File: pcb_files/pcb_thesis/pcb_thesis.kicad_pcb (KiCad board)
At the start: 2 copper layers, 22 parts, among them J1 goldpin 1x6, J2 goldpin 1x2, J3 goldpin 1x2, Q1 PNP, SW1 RESET SW, SW3 ACTION SW, U1 ATmega32L-8AU, Y1 8MHz

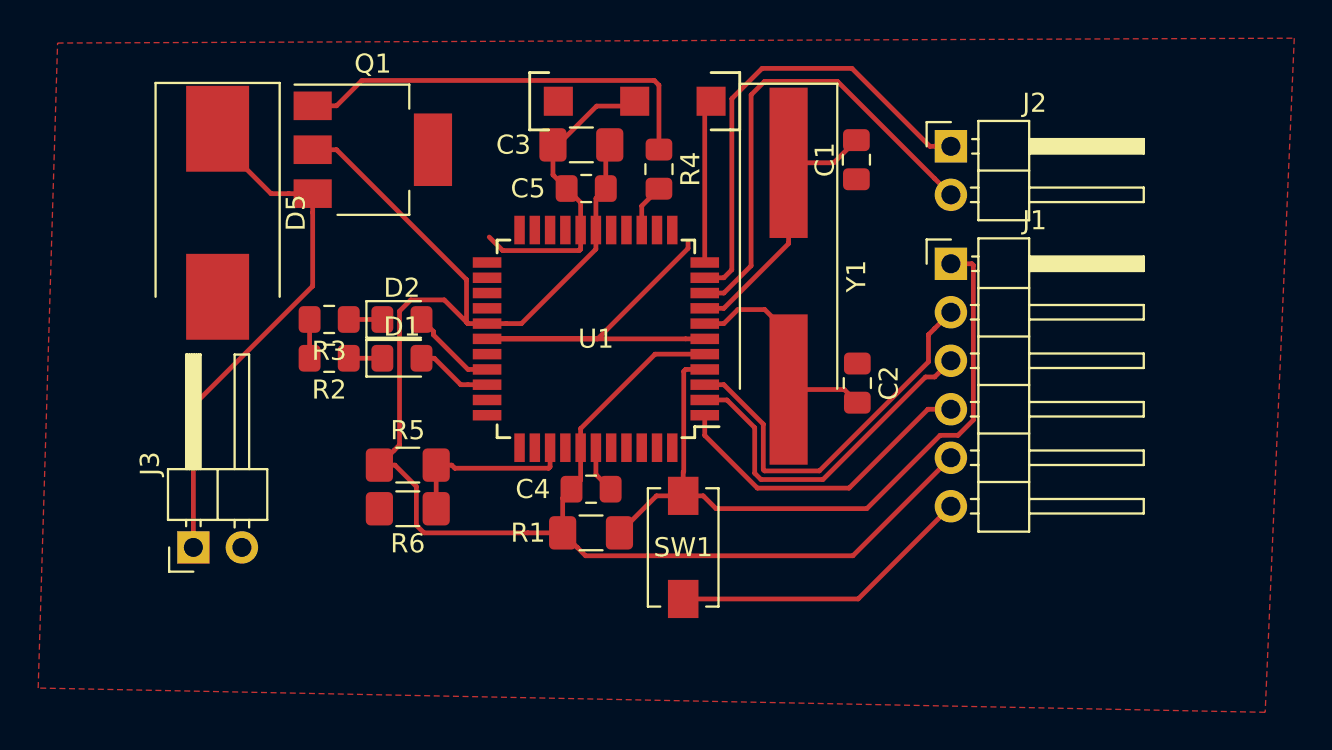
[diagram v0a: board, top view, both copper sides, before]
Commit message: Przygotowanie plikow do wytrawiania plytki
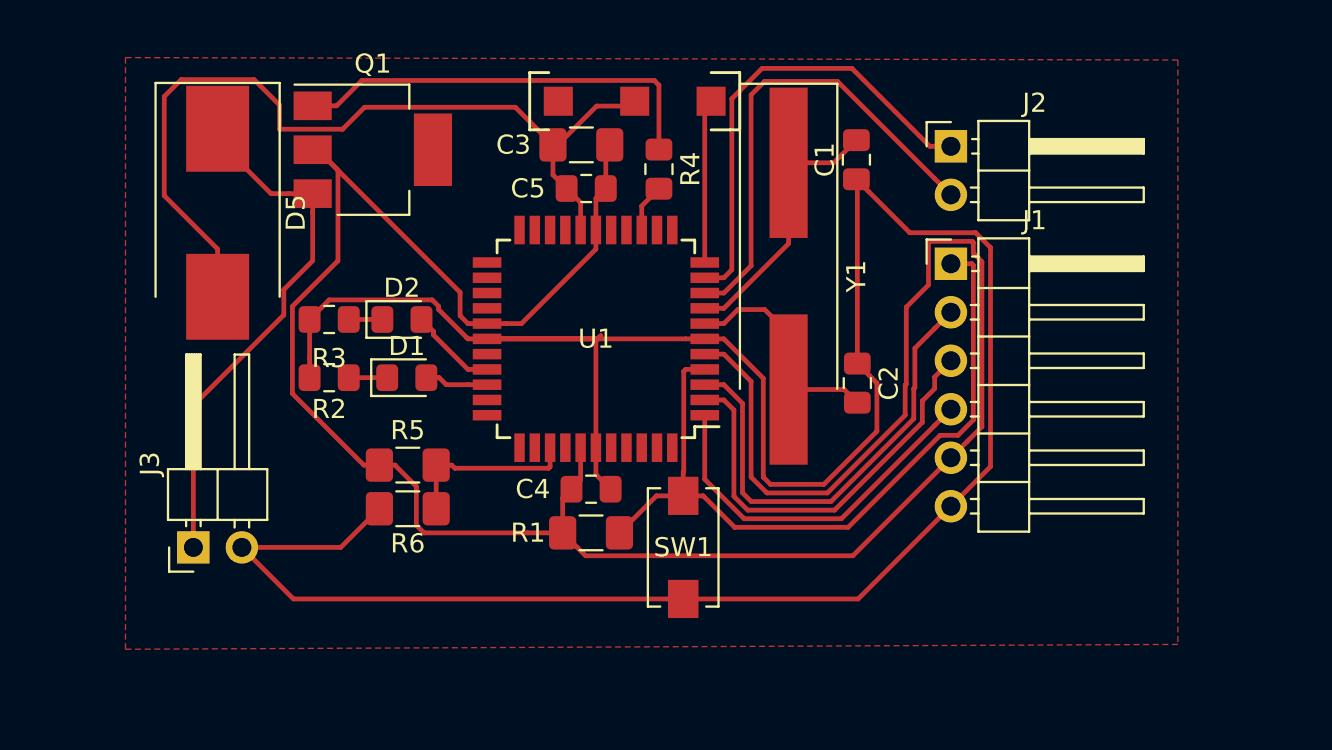
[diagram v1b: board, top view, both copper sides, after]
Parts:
- moved D1 1.05 mm to (130.3, 77.2)
- moved R2 1.02 mm to (126.2, 77.2)
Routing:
- net GND: track 60.9 -> 186.4 mm
- net VCC: track 89.1 -> 129.0 mm
- net Net-(J1-Pad2): track 20.4 -> 24.4 mm
- net Net-(J1-Pad3): track 18.6 -> 22.2 mm
- net Net-(J1-Pad4): track 16.8 -> 19.5 mm
- net /~RESET: track 38.5 -> 39.3 mm
- net Net-(D1-Pad2): track 4.01 -> 3.33 mm

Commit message: Added all pcb files
Mysle ze to wszystkie juz... i nie bedzie zmian.
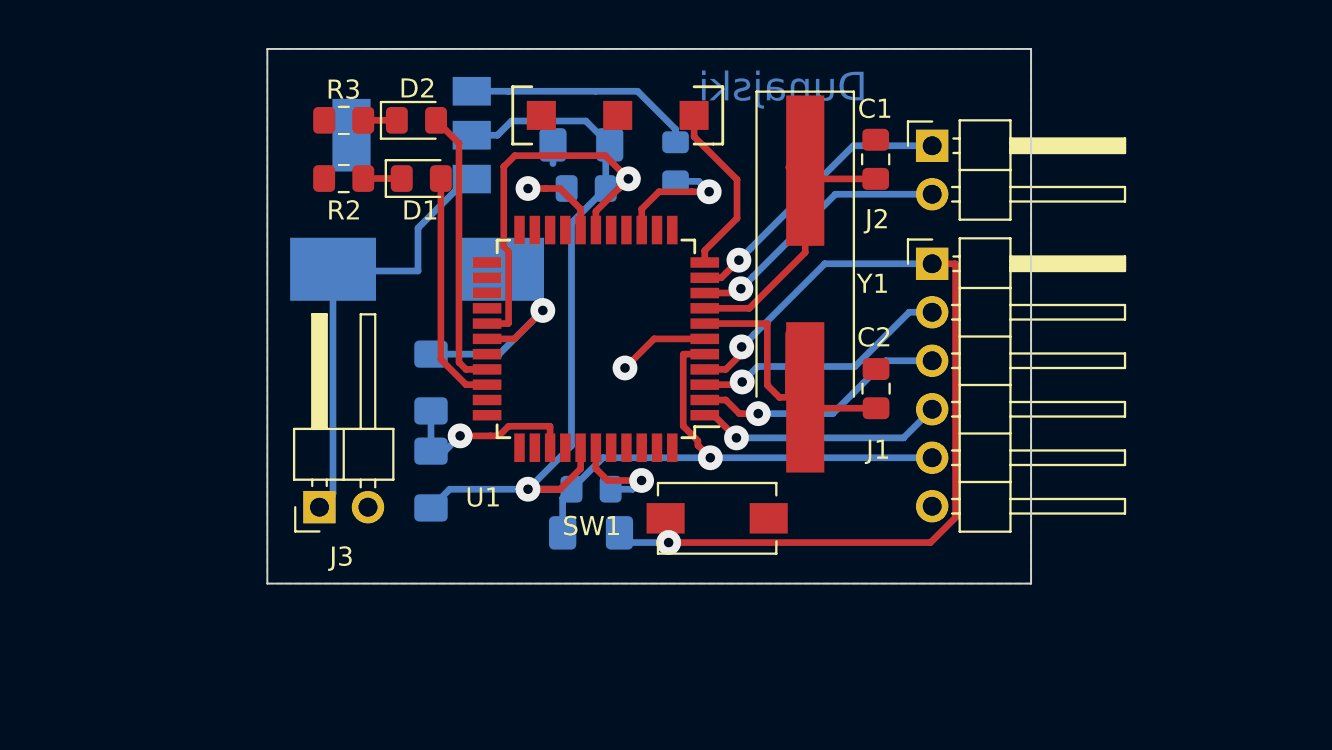
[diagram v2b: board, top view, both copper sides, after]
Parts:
- C3, C4, C5, D5, Q1, R1, R4, R5, R6: moved to B.Cu
- moved D5 10.9 mm to (130.8, 71.5), turned to 0 degrees
- moved D2 10.5 mm to (130.8, 63.7)
- moved R3 10.5 mm to (127.0, 63.7)
- moved D1 10.5 mm to (131.1, 66.8)
- moved R2 10.5 mm to (127.0, 66.8)
- moved J3 6.93 mm to (125.7, 84.0)
- moved R6 6.72 mm to (131.6, 77.5), turned to 90 degrees
- moved SW1 2.34 mm to (146.6, 84.6), turned to 180 degrees
- moved Q1 2.17 mm to (130.6, 64.5), turned to 180 degrees
- moved R5 1.43 mm to (131.6, 82.5), turned to 90 degrees
- moved SW3 1.16 mm to (141.3, 63.5)
- moved C2 1.02 mm to (154.9, 77.8)
- moved C1 1.01 mm to (154.9, 65.8), turned to 270 degrees
- moved J2 0.98 mm to (157.8, 65.1)
- moved J1 0.98 mm to (157.8, 71.2)
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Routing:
- net GND: track 186.4 -> 26.5 mm, vias 0 -> 4
- net VCC: track 129.0 -> 91.1 mm, vias 0 -> 3
- net Net-(J2-Pad2): track 25.2 -> 14.1 mm, vias 0 -> 1
- net Net-(J1-Pad2): track 24.4 -> 13.9 mm, vias 0 -> 1
- net Net-(D2-Pad2): track 4.62 -> 14.8 mm
- net Net-(Q1-Pad1): track 22.2 -> 12.2 mm
- net Net-(J2-Pad1): track 24.4 -> 14.8 mm, vias 0 -> 1
- net /~RESET: track 39.3 -> 48.7 mm, vias 0 -> 2
- net Net-(D1-Pad2): track 3.33 -> 12.4 mm
- net Net-(J1-Pad3): track 22.2 -> 13.4 mm, vias 0 -> 1
- net Net-(J1-Pad4): track 19.5 -> 13.0 mm, vias 0 -> 1
- net Net-(D5-Pad1): track 27.9 -> 21.5 mm
- net Net-(C2-Pad2): track 12.0 -> 17.5 mm
- net /PWM_M: track 2.54 -> 6.99 mm, vias 0 -> 1
- net Net-(C1-Pad2): track 14.1 -> 15.5 mm
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- added copper zone on B.Cu, net GND
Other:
- board outline added: 40 x 28 mm
- net class wszystkie added: clearance 0.2, trace_width 0.35, via_dia 1.3, via_drill 0.5
- rule pad_to_mask_clearance: 0 -> 0.1
- board text added: "Dunajski"
